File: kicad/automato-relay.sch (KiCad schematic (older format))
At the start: 34 parts, among them J1 TE-3-213598-4, J2 Screw_Terminal_01x03, J3 TE-3-213598-4, J4 Screw_Terminal_01x05, J5 TE-3-213598-4, J6 TE-3-213598-4, J7 Screw_Terminal_01x04, J8 TE-3-213598-4, K1 G5LE-14, K2 G5LE-14, K3 G5LE-14, K4 G5LE-14, Q1 DMG3418L, Q2 DMG3418L, Q3 DMG3418L, Q4 DMG3418L, U1 74HC595

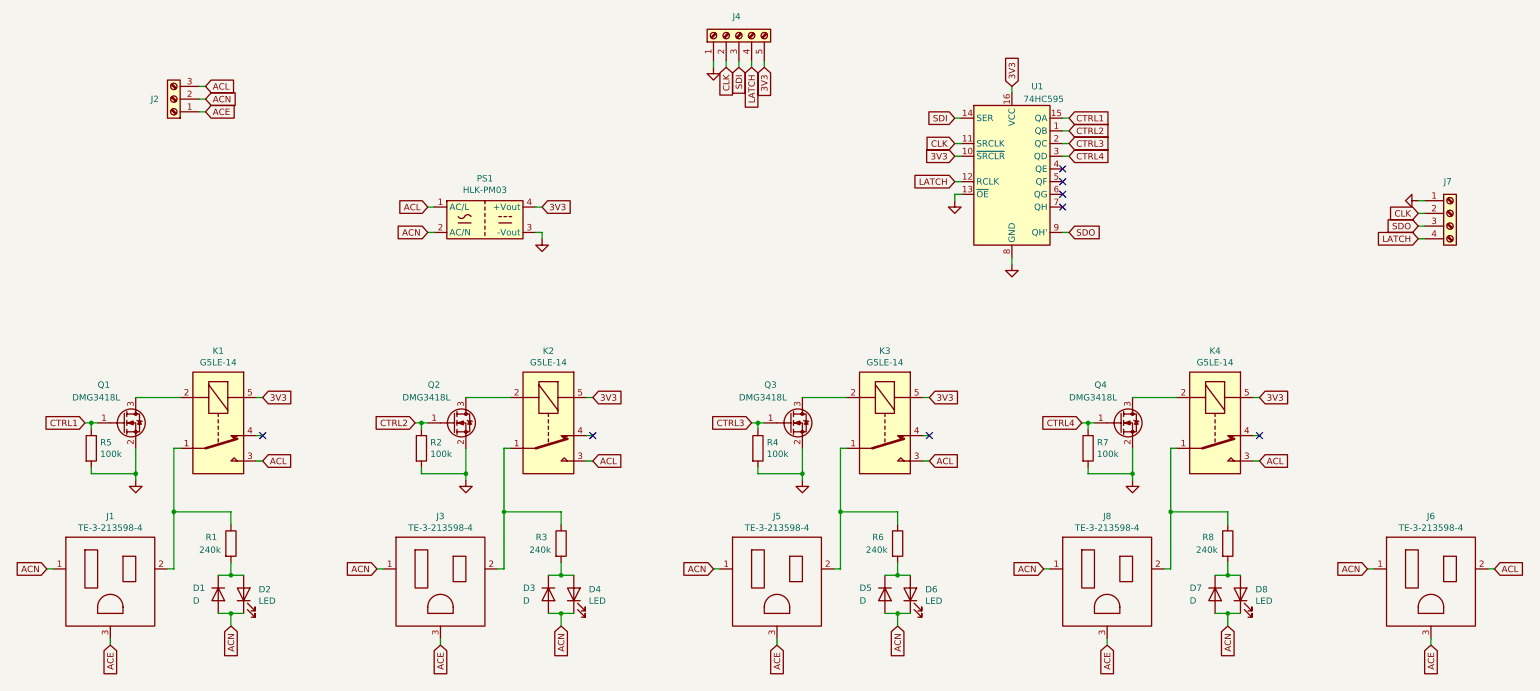
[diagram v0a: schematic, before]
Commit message: All traces routed
MOV added, 10 hours in.  Final approval of layout.  Power planes to pour.
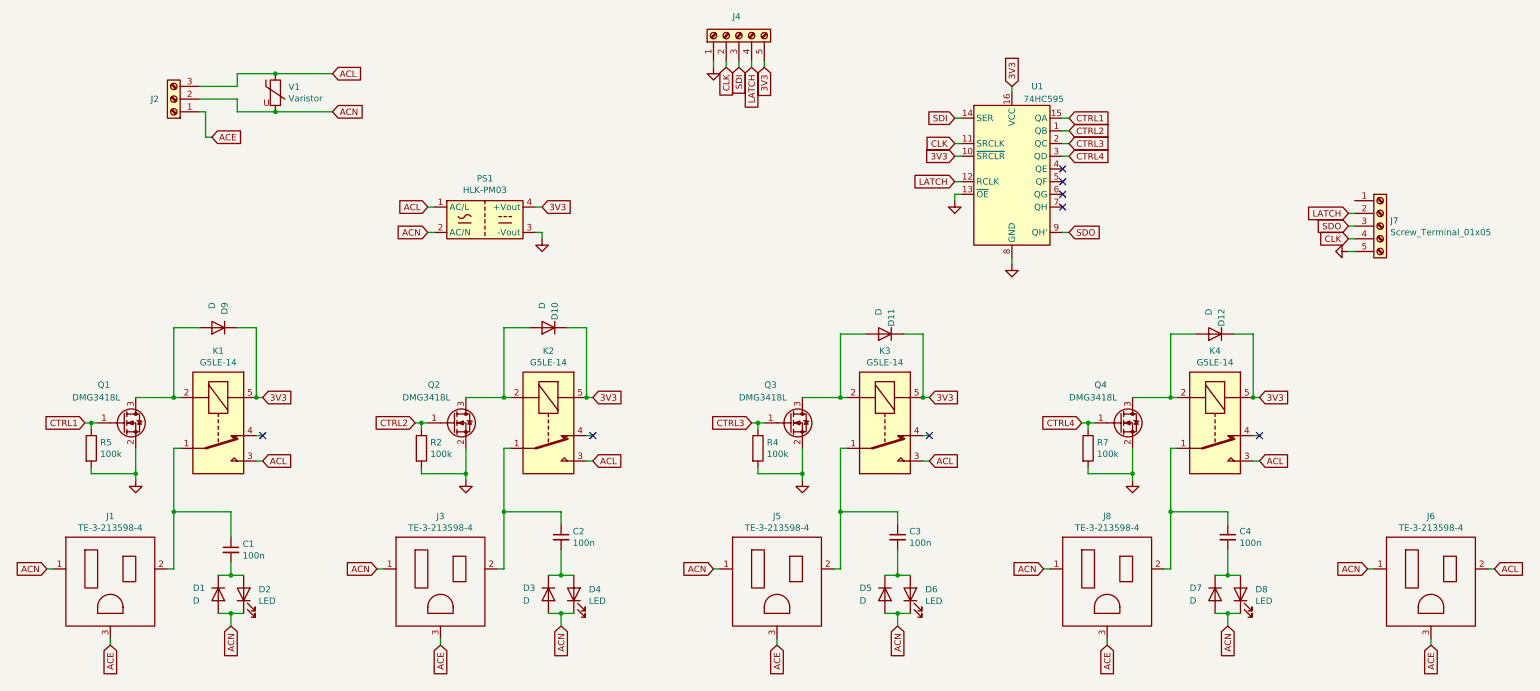
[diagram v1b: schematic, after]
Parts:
- removed J7: Screw_Terminal_01x04, symbol Connector:Screw_Terminal_01x04
- removed R1, R3, R6, R8: 240k, symbol Device:R
- added C1, C2, C3, C4: 100n, Capacitor_SMD:C_1206_3216Metric, symbol Device:C_Small
- added D10, D11, D12, D9: D, Diode_SMD:D_SOT-23_ANK, symbol Device:D
- added J7: Screw_Terminal_01x05, Connector_Phoenix_MC_HighVoltage:PhoenixContact_MC_1,5_5-G-5.08_1x05_P5.08mm_Horizontal, symbol Connector:Screw_Terminal_01x05
- added V1: Varistor, Varistor:RV_Disc_D7mm_W3.5mm_P5mm, symbol Device:Varistor
- D1, D3, D5, D7: footprint (none) -> Diode_SMD:D_SOT-23_ANK
- D2, D4, D6, D8: footprint (none) -> LED_SMD:LED_1206_3216Metric
- J1, J3, J5, J6, J8: footprint (none) -> automato-relay:TE-3-213598-4
- J2: footprint (none) -> Connector_Phoenix_MC_HighVoltage:PhoenixContact_MCV_1,5_3-G-5.08_1x03_P5.08mm_Vertical
- J4: footprint (none) -> Connector_Phoenix_MC_HighVoltage:PhoenixContact_MC_1,5_5-G-5.08_1x05_P5.08mm_Horizontal
- R2, R4, R5, R7: footprint (none) -> Resistor_SMD:R_0805_2012Metric
- U1: footprint (none) -> Package_SO:SO-16_3.9x9.9mm_P1.27mm
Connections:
- net 3V3: now also D10.1 (K), D11.1 (K), D12.1 (K), D9.1 (K)
- net ACL: now also V1.1
- net ACN: now also V1.2
- net CLK: now also J7.4 (Pin_4)
- net GND: now also J7.5 (Pin_5)
- net LATCH: now also J7.2 (Pin_2)
- net SDO: now also J7.3 (Pin_3)
- net at J1.2 (Hot), K1.1: now also C1.1
- net at K1.2, Q1.3 (D): now also D9.2 (A)
- net at D1.1 (K), D2.2 (A): now also C1.2
- net at J3.2 (Hot), K2.1: now also C2.1
- net at K2.2, Q2.3 (D): now also D10.2 (A)
- net at D3.1 (K), D4.2 (A): now also C2.2
- net at J5.2 (Hot), K3.1: now also C3.1
- net at K3.2, Q3.3 (D): now also D11.2 (A)
- net at D5.1 (K), D6.2 (A): now also C3.2
- net at J8.2 (Hot), K4.1: now also C4.1
- net at K4.2, Q4.3 (D): now also D12.2 (A)
- net at D7.1 (K), D8.2 (A): now also C4.2
